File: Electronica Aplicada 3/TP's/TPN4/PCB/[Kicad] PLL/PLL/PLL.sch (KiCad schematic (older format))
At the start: 26 parts, among them J1 Alimentacion, J2 SeñalDeReferencia, SW1 SW_SPDT, U1 4017, U2 4046

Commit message: arreglo error PLL y actualizo valores
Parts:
- removed SW1: SW_SPDT, lib_fp:PinHeader_1x03_P2.54mm_Vertical, symbol Switch:SW_SPDT
- C1: value 100n -> 330p; symbol Device:C_Small -> PLL-rescue:C_Small-Device
- C2, C5: symbol Device:C_Small -> PLL-rescue:C_Small-Device
- C3, C6: symbol Device:CP1_Small -> PLL-rescue:CP1_Small-Device
- C4: value 680p -> 0p; symbol Device:C_Variable -> PLL-rescue:C_Variable-Device
- C7: value 680n -> 100n; symbol Device:C_Small -> PLL-rescue:C_Small-Device
- C8: value 680n -> 100n; symbol Device:C_Variable -> PLL-rescue:C_Variable-Device
- D1, D2: symbol Device:LED -> PLL-rescue:LED-Device
- J1, J2: symbol Connector:Screw_Terminal_01x02 -> PLL-rescue:Screw_Terminal_01x02-Connector
- R1, R2, R3, R4, R5, R6: symbol Device:R_US -> PLL-rescue:R_US-Device
- RV1, RV2, RV3: symbol Device:R_POT_TRIM_US -> PLL-rescue:R_POT_TRIM_US-Device
- TP1, TP2: symbol Connector:TestPoint_Probe -> PLL-rescue:TestPoint_Probe-Connector
- U1: symbol 4xxx:4017 -> PLL-rescue:4017-4xxx
- U2: symbol 4xxx:4046 -> PLL-rescue:4046-4xxx
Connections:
- wire segments 83 -> 76
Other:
- note added: "27k"
- note added: "48k"
- note added: "50"

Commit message: Actualizo
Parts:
- added Q1: BC337, lib_fp:TO-92_Inline, symbol PLL_sch:BC337
- added R7: 100, lib_fp:R_Axial_DIN0207_L6.3mm_D2.5mm_P10.16mm_Horizontal, symbol PLL_sch:R_US
- added R8: 10k, lib_fp:R_Axial_DIN0207_L6.3mm_D2.5mm_P10.16mm_Horizontal, symbol PLL_sch:R_US
- C1, C2, C5, C7: symbol PLL-rescue:C_Small-Device -> PLL_sch:C_Small
- C3, C6: symbol PLL-rescue:CP1_Small-Device -> PLL_sch:CP1_Small
- C4, C8: symbol PLL-rescue:C_Variable-Device -> PLL_sch:C_Variable
- D1, D2: symbol PLL-rescue:LED-Device -> PLL_sch:LED
- J1, J2: symbol PLL-rescue:Screw_Terminal_01x02-Connector -> PLL_sch:Screw_Terminal_01x02
- R1, R2, R3, R4, R5, R6: symbol PLL-rescue:R_US-Device -> PLL_sch:R_US
- RV1, RV2, RV3: symbol PLL-rescue:R_POT_TRIM_US-Device -> PLL_sch:R_POT_TRIM_US
- TP1, TP2: symbol PLL-rescue:TestPoint_Probe-Connector -> PLL_sch:TestPoint_Probe
- U1: symbol PLL-rescue:4017-4xxx -> PLL_sch:4017
- U2: symbol PLL-rescue:4046-4xxx -> PLL_sch:4046
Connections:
- net +12V: now also R8.1
- net GND: now also Q1.3 (E)
- net f_in: now also Q1.1 (C), R8.2; no longer J2.2 (Pin_2)
- new net: Q1.2 (B), R7.2
- new net generador: J2.2 (Pin_2), R7.1
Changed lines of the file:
@@
 $EndDescr
 $Comp
-L PLL-rescue:4017-4xxx U1
+L PLL_sch:4017 U1
 U 1 1 5D03BE37
 P 4025 4250
@@
 $EndComp
 $Comp
-L PLL-rescue:R_US-Device R1
+L PLL_sch:R_US R1
 U 1 1 5D03DC80
 P 5400 5050
@@
 $EndComp
 $Comp
-L PLL-rescue:LED-Device D1
+L PLL_sch:LED D1
 U 1 1 5D03FB9E
 P 2750 4575
@@
 $EndComp
 $Comp
-L PLL-rescue:GND-power #PWR09
+L PLL_sch:GND #PWR09
 U 1 1 5D0464B6
 P 4025 5200
@@
 	4025 5200 4025 5150
 $Comp
-L PLL-rescue:+12V-power #PWR08
+L PLL_sch:+12V #PWR08
 U 1 1 5D04819C
 P 4025 3225
@@
 $EndComp
 $Comp
-L PLL-rescue:CP1_Small-Device C3
+L PLL_sch:CP1_Small C3
 U 1 1 5D048F94
 P 4150 3375
@@
 Connection ~ 4025 3275
 $Comp
-L PLL-rescue:GND-power #PWR010
+L PLL_sch:GND #PWR010
 U 1 1 5D049AB6
 P 4150 3475
@@
 	4025 3225 4025 3275
 $Comp
-L PLL-rescue:C_Small-Device C2
+L PLL_sch:C_Small C2
 U 1 1 5D04AB9C
 P 3875 3375
@@
 	4025 3275 3875 3275
 $Comp
-L PLL-rescue:GND-power #PWR07
+L PLL_sch:GND #PWR07
 U 1 1 5D04BC49
 P 3875 3475
@@
 $EndComp
 $Comp
-L PLL-rescue:GND-power #PWR016
+L PLL_sch:GND #PWR016
 U 1 1 5D04CA1A
 P 6600 5275
@@
 	5550 4400 5550 4700
 $Comp
-L PLL-rescue:GND-power #PWR011
+L PLL_sch:GND #PWR011
 U 1 1 5D050E57
 P 5400 5275
@@
 	6600 5275 6600 5000
 $Comp
-L PLL-rescue:+12V-power #PWR015
+L PLL_sch:+12V #PWR015
 U 1 1 5D053CE4
 P 6600 3275
@@
 $EndComp
 $Comp
-L PLL-rescue:CP1_Small-Device C6
+L PLL_sch:CP1_Small C6
 U 1 1 5D053CEA
 P 6725 3425
@@
 	6600 3275 6600 3325
 $Comp
-L PLL-rescue:C_Small-Device C5
+L PLL_sch:C_Small C5
 U 1 1 5D053CF3
 P 6450 3425
@@
 	6600 3325 6450 3325
 $Comp
-L PLL-rescue:GND-power #PWR014
+L PLL_sch:GND #PWR014
 U 1 1 5D053EF9
 P 6450 3525
@@
 $EndComp
 $Comp
-L PLL-rescue:GND-power #PWR017
+L PLL_sch:GND #PWR017
 U 1 1 5D054535
 P 6725 3525
@@
 $EndComp
 $Comp
-L PLL-rescue:+12V-power #PWR04
+L PLL_sch:+12V #PWR04
 U 1 1 5D05567F
 P 2750 3975
@@
 $EndComp
 $Comp
-L PLL-rescue:R_US-Device R3
+L PLL_sch:R_US R3
 U 1 1 5D05685E
 P 2750 4200
@@
 	4525 4850 5100 4850
 $Comp
-L PLL-rescue:Screw_Terminal_01x02-Connector J2
+L PLL_sch:Screw_Terminal_01x02 J2
 U 1 1 5D05FA70
 P 1925 3525
@@
 	1725 3425 1575 3425
 $Comp
-L PLL-rescue:GND-power #PWR03
+L PLL_sch:GND #PWR03
 U 1 1 5D0619A8
 P 1650 3575
@@
 	1650 3525 1725 3525
 $Comp
-L PLL-rescue:Screw_Terminal_01x02-Connector J1
+L PLL_sch:Screw_Terminal_01x02 J1
 U 1 1 5D063274
 P 1900 4000
@@
 	1700 4000 1625 4000
 $Comp
-L PLL-rescue:GND-power #PWR02
+L PLL_sch:GND #PWR02
 U 1 1 5D06327C
 P 1625 4150
@@
 	1625 4100 1700 4100
 $Comp
-L PLL-rescue:+12V-power #PWR01
+L PLL_sch:+12V #PWR01
 U 1 1 5D0635E3
 P 1625 4000
@@
 	1    0    0    -1
 $EndComp
-Text GLabel 1575 3425 0    50   Input ~ 0
-f_in
 Text GLabel 5975 3900 0    50   Input ~ 0
 f_in
 $Comp
-L PLL-rescue:TestPoint_Probe-Connector TP2
+L PLL_sch:TestPoint_Probe TP2
 U 1 1 5D066A8E
 P 7175 3800
@@
 	7100 3800 7175 3800
 $Comp
-L PLL-rescue:R_US-Device R6
+L PLL_sch:R_US R6
 U 1 1 5D06D844
 P 8625 4150
@@
 $EndComp
 $Comp
-L PLL-rescue:GND-power #PWR020
+L PLL_sch:GND #PWR020
 U 1 1 5D06FD70
 P 8625 4700
@@
 	3175 3750 3525 3750
 $Comp
-L PLL-rescue:GND-power #PWR06
+L PLL_sch:GND #PWR06
 U 1 1 5D072DC3
 P 3425 4175
@@
 	3425 4050 3425 4175
 $Comp
-L PLL-rescue:GND-power #PWR013
+L PLL_sch:GND #PWR013
 U 1 1 5D074D13
 P 6075 5275
@@
 	6075 4700 6100 4700
 $Comp
-L PLL-rescue:R_US-Device R4
+L PLL_sch:R_US R4
 U 1 1 5D076D70
 P 7275 4750
@@
 	7275 4500 7100 4500
 $Comp
-L PLL-rescue:GND-power #PWR018
+L PLL_sch:GND #PWR018
 U 1 1 5D07906B
 P 7275 5275
@@
 	7100 4200 7500 4200
 $Comp
-L PLL-rescue:C_Small-Device C1
+L PLL_sch:C_Small C1
 U 1 1 5D08B1EA
 P 5950 4150
@@
 	6100 4200 6100 4250
 $Comp
-L PLL-rescue:LED-Device D2
+L PLL_sch:LED D2
 U 1 1 5D091A36
 P 8050 4900
@@
 $EndComp
 $Comp
-L PLL-rescue:GND-power #PWR019
+L PLL_sch:GND #PWR019
 U 1 1 5D091A3C
 P 8075 5075
@@
 $EndComp
 $Comp
-L PLL-rescue:R_US-Device R5
+L PLL_sch:R_US R5
 U 1 1 5D091A42
 P 8050 4575
@@
 	7100 4400 8050 4400
 $Comp
-L PLL-rescue:TestPoint_Probe-Connector TP1
+L PLL_sch:TestPoint_Probe TP1
 U 1 1 5D0A9B68
 P 3075 4775
@@
 $EndComp
 $Comp
-L PLL-rescue:GND-power #PWR05
+L PLL_sch:GND #PWR05
 U 1 1 5D0AF46A
 P 2750 4825
@@
 	5600 4000 5950 4000
 $Comp
-L PLL-rescue:C_Variable-Device C4
+L PLL_sch:C_Variable C4
 U 1 1 5D0BC112
 P 5600 4150
@@
 	5950 4300 5600 4300
 $Comp
-L PLL-rescue:R_POT_TRIM_US-Device RV1
+L PLL_sch:R_POT_TRIM_US RV1
 U 1 1 5D0CD8E8
 P 5400 4700
@@
 	5400 5275 5400 5200
 $Comp
-L PLL-rescue:R_POT_TRIM_US-Device RV2
+L PLL_sch:R_POT_TRIM_US RV2
 U 1 1 5D0DB87B
 P 5775 4700
@@
 	5925 4500 6100 4500
 $Comp
-L PLL-rescue:R_US-Device R2
+L PLL_sch:R_US R2
 U 1 1 5D0E711A
 P 5775 5050
@@
 $EndComp
 $Comp
-L PLL-rescue:GND-power #PWR012
+L PLL_sch:GND #PWR012
 U 1 1 5D0E7949
 P 5775 5275
@@
 	5775 5275 5775 5200
 $Comp
-L PLL-rescue:R_POT_TRIM_US-Device RV3
+L PLL_sch:R_POT_TRIM_US RV3
 U 1 1 5D0E9A55
 P 8300 4000
@@
 	7500 4300 7500 4200
 $Comp
-L PLL-rescue:C_Variable-Device C8
+L PLL_sch:C_Variable C8
 U 1 1 5D1148E7
 P 8875 4450
@@
 	8625 4600 8625 4550
 $Comp
-L PLL-rescue:C_Small-Device C7
+L PLL_sch:C_Small C7
 U 1 1 5D06E1B8
 P 8625 4450
@@
 	6600 3325 6600 3500
 $Comp
-L PLL-rescue:4046-4xxx U2
+L PLL_sch:4046 U2
 U 1 1 5D04140C
 P 6600 4200
@@
 	7100 4000 8100 4000
 Connection ~ 8100 4000
+$Comp
+L PLL_sch:BC337 Q1
+U 1 1 5D069771
+P 2650 5900
+F 0 "Q1" H 2841 5946 50  0000 L CNN
+F 1 "BC337" H 2841 5855 50  0000 L CNN
+F 2 "lib_fp:TO-92_Inline" H 2850 5825 50  0001 L CIN
+F 3 "https://diotec.com/tl_files/diotec/files/pdf/datasheets/bc337.pdf" H 2650 5900 50  0001 L CNN
+	1    2650 5900
+	1    0    0    -1
+$EndComp
+$Comp
+L PLL_sch:+12V #PWR0101
+U 1 1 5D06BD1F
+P 2750 5250
+F 0 "#PWR0101" H 2750 5100 50  0001 C CNN
+F 1 "+12V" H 2764 5419 50  0000 C CNN
+F 2 "" H 2750 5250 50  0001 C CNN
+F 3 "" H 2750 5250 50  0001 C CNN
+	1    2750 5250
+	1    0    0    -1
+$EndComp
+Wire Wire Line
+	2750 5250 2750 5300
+$Comp
+L PLL_sch:R_US R8
+U 1 1 5D06F998
+P 2750 5450
+F 0 "R8" H 2825 5500 50  0000 L CNN
+F 1 "10k" H 2825 5400 50  0000 L CNN
+F 2 "lib_fp:R_Axial_DIN0207_L6.3mm_D2.5mm_P10.16mm_Horizontal" V 2790 5440 50  0001 C CNN
+F 3 "~" H 2750 5450 50  0001 C CNN
+	1    2750 5450
+	1    0    0    -1
+$EndComp
+$Comp
+L PLL_sch:R_US R7
+U 1 1 5D070556
+P 2150 5900
+F 0 "R7" V 2250 5850 50  0000 L CNN
+F 1 "100" V 2050 5850 50  0000 L CNN
+F 2 "lib_fp:R_Axial_DIN0207_L6.3mm_D2.5mm_P10.16mm_Horizontal" V 2190 5890 50  0001 C CNN
+F 3 "~" H 2150 5900 50  0001 C CNN
+	1    2150 5900
+	0    -1   -1   0
+$EndComp
+Wire Wire Line
+	2300 5900 2450 5900
+$Comp
+L PLL_sch:GND #PWR0102
+U 1 1 5D073650
+P 2750 6200
+F 0 "#PWR0102" H 2750 5950 50  0001 C CNN
+F 1 "GND" H 2754 6032 50  0000 C CNN
+F 2 "" H 2750 6200 50  0001 C CNN
+F 3 "" H 2750 6200 50  0001 C CNN
+	1    2750 6200
+	1    0    0    -1
+$EndComp
+Wire Wire Line
+	2750 6200 2750 6100
+Text GLabel 1900 5900 0    50   Input ~ 0
+generador
+Wire Wire Line
+	1900 5900 2000 5900
+Wire Wire Line
+	2750 5600 2750 5700
+Wire Wire Line
+	2750 5700 3150 5700
+Connection ~ 2750 5700
+Text GLabel 3150 5700 2    50   Output ~ 0
+f_in
+Text GLabel 1575 3425 0    50   Input ~ 0
+generador
 $EndSCHEMATC

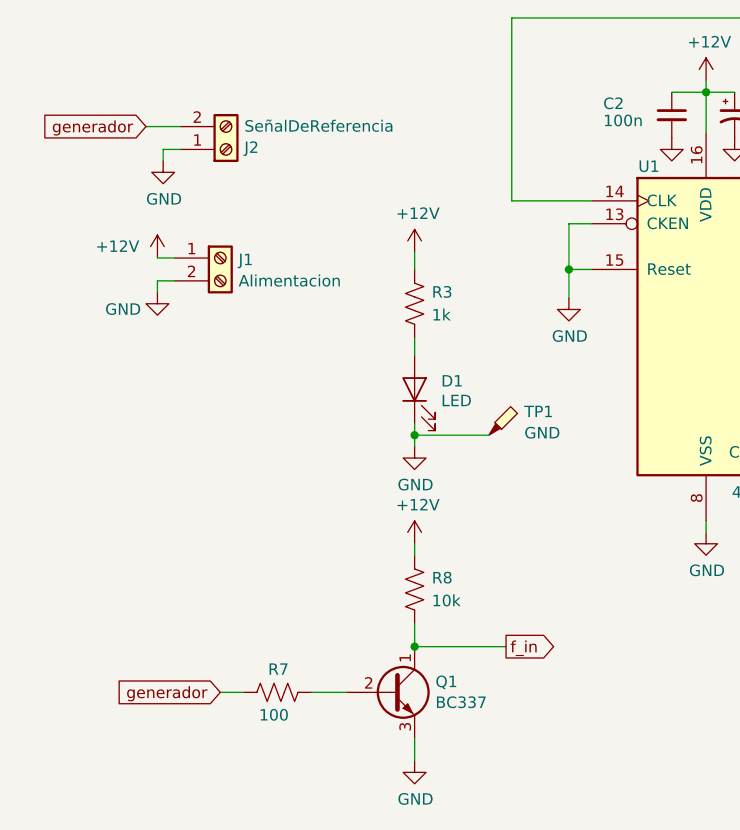
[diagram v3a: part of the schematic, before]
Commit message: PLL
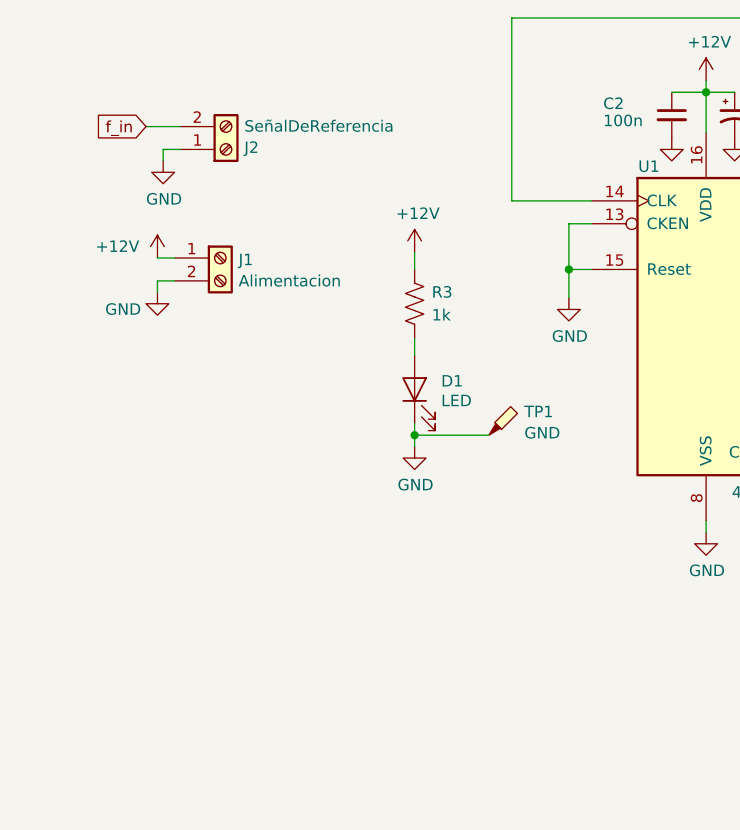
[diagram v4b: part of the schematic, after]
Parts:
- removed Q1: BC337, lib_fp:TO-92_Inline, symbol PLL_sch:BC337
- removed R7: 100, lib_fp:R_Axial_DIN0207_L6.3mm_D2.5mm_P10.16mm_Horizontal, symbol PLL_sch:R_US
- removed R8: 10k, lib_fp:R_Axial_DIN0207_L6.3mm_D2.5mm_P10.16mm_Horizontal, symbol PLL_sch:R_US
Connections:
- net generador is gone; now on net f_in: J2.2 (Pin_2)
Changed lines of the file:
@@
 	7100 4000 8100 4000
 Connection ~ 8100 4000
-$Comp
-L PLL_sch:BC337 Q1
-U 1 1 5D069771
-P 2650 5900
-F 0 "Q1" H 2841 5946 50  0000 L CNN
-F 1 "BC337" H 2841 5855 50  0000 L CNN
-F 2 "lib_fp:TO-92_Inline" H 2850 5825 50  0001 L CIN
-F 3 "https://diotec.com/tl_files/diotec/files/pdf/datasheets/bc337.pdf" H 2650 5900 50  0001 L CNN
-	1    2650 5900
-	1    0    0    -1
-$EndComp
-$Comp
-L PLL_sch:+12V #PWR0101
-U 1 1 5D06BD1F
-P 2750 5250
-F 0 "#PWR0101" H 2750 5100 50  0001 C CNN
-F 1 "+12V" H 2764 5419 50  0000 C CNN
-F 2 "" H 2750 5250 50  0001 C CNN
-F 3 "" H 2750 5250 50  0001 C CNN
-	1    2750 5250
-	1    0    0    -1
-$EndComp
-Wire Wire Line
-	2750 5250 2750 5300
-$Comp
-L PLL_sch:R_US R8
-U 1 1 5D06F998
-P 2750 5450
-F 0 "R8" H 2825 5500 50  0000 L CNN
-F 1 "10k" H 2825 5400 50  0000 L CNN
-F 2 "lib_fp:R_Axial_DIN0207_L6.3mm_D2.5mm_P10.16mm_Horizontal" V 2790 5440 50  0001 C CNN
-F 3 "~" H 2750 5450 50  0001 C CNN
-	1    2750 5450
-	1    0    0    -1
-$EndComp
-$Comp
-L PLL_sch:R_US R7
-U 1 1 5D070556
-P 2150 5900
-F 0 "R7" V 2250 5850 50  0000 L CNN
-F 1 "100" V 2050 5850 50  0000 L CNN
-F 2 "lib_fp:R_Axial_DIN0207_L6.3mm_D2.5mm_P10.16mm_Horizontal" V 2190 5890 50  0001 C CNN
-F 3 "~" H 2150 5900 50  0001 C CNN
-	1    2150 5900
-	0    -1   -1   0
-$EndComp
-Wire Wire Line
-	2300 5900 2450 5900
-$Comp
-L PLL_sch:GND #PWR0102
-U 1 1 5D073650
-P 2750 6200
-F 0 "#PWR0102" H 2750 5950 50  0001 C CNN
-F 1 "GND" H 2754 6032 50  0000 C CNN
-F 2 "" H 2750 6200 50  0001 C CNN
-F 3 "" H 2750 6200 50  0001 C CNN
-	1    2750 6200
-	1    0    0    -1
-$EndComp
-Wire Wire Line
-	2750 6200 2750 6100
-Text GLabel 1900 5900 0    50   Input ~ 0
-generador
-Wire Wire Line
-	1900 5900 2000 5900
-Wire Wire Line
-	2750 5600 2750 5700
-Wire Wire Line
-	2750 5700 3150 5700
-Connection ~ 2750 5700
-Text GLabel 3150 5700 2    50   Output ~ 0
+Text GLabel 1575 3425 0    50   Input ~ 0
 f_in
-Text GLabel 1575 3425 0    50   Input ~ 0
-generador
 $EndSCHEMATC
